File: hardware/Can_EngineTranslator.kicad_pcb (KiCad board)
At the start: 2 copper layers, 72 x 63 mm, 63 parts, among them J1 ProgramerConnector, J2 CANcarConnector, J3 CANinverterConnector, J5 PowerOutputConnector, Q1 BSS138, SW1 SW_Push, U1 STM32F105RBTx, U2 LM2596S-5, U3 LM1117-3.3, U4 MCP2562-H-SN, U5 MCP2562-H-SN, Y1 Crystal 8 MHz

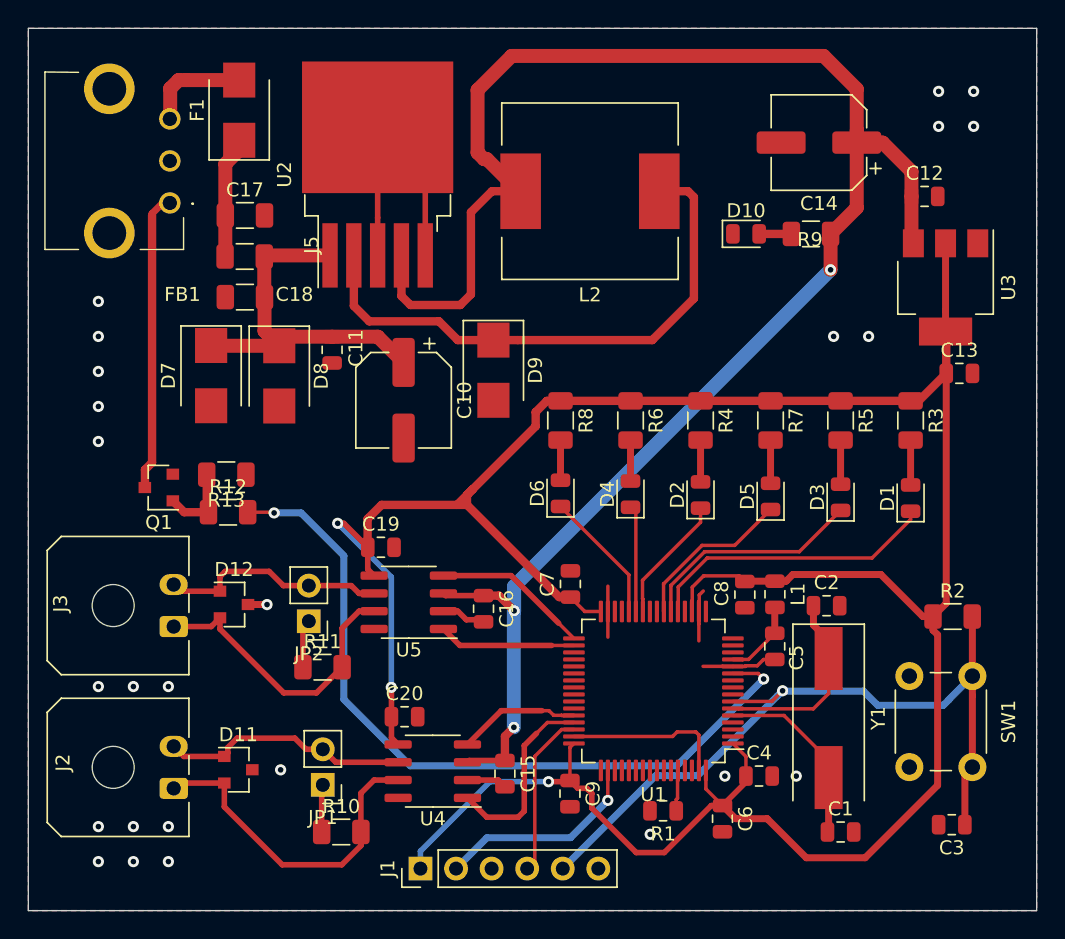
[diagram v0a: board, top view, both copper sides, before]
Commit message: Cosmetic changes to pcb
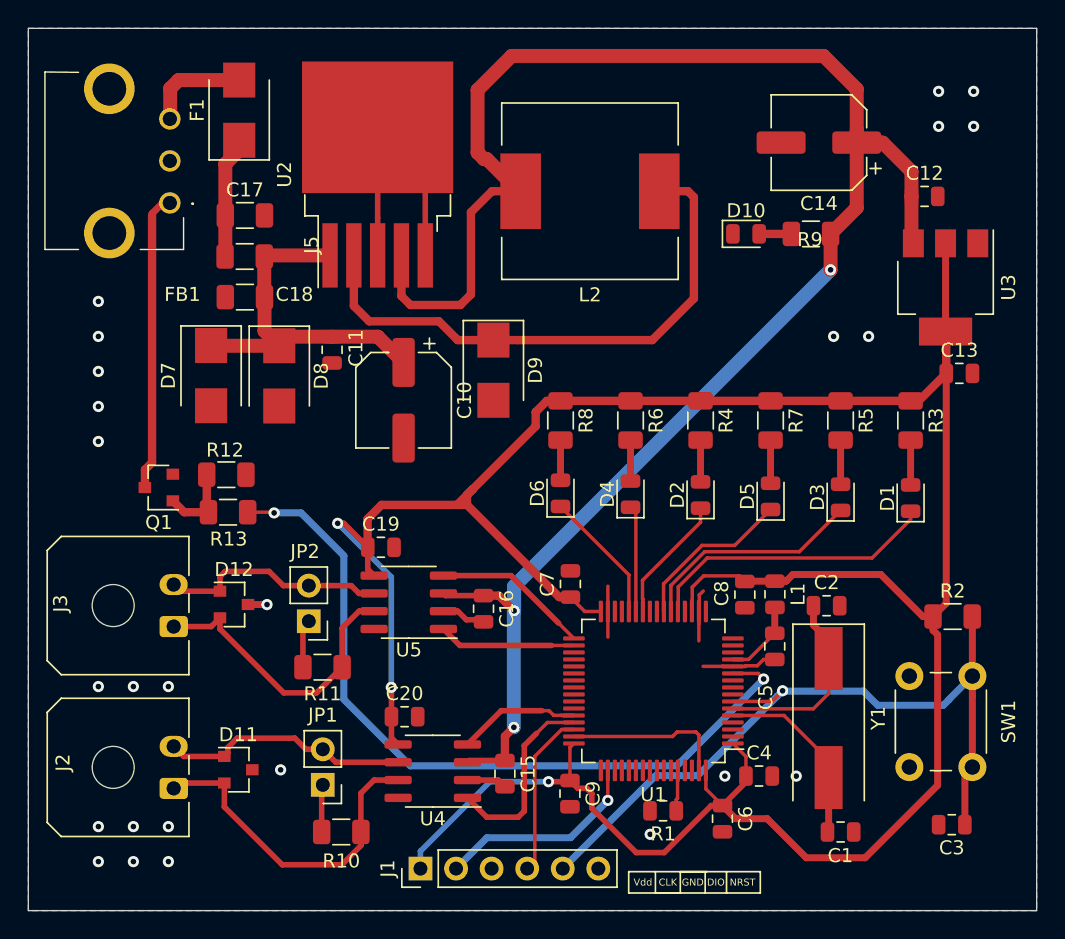
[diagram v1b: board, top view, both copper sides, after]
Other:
- board text added: "CLK"
- board text added: "DIO"
- board text added: "GND"
- board text added: "NRST"
- board text added: "Vdd"
